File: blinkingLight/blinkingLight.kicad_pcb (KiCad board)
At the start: 2 copper layers, 50.8 x 50.8 mm, 11 parts, among them J1 Conn_02x03_Odd_Even, J2 Conn_01x02_Pin, Q1 BC548, U1 ICM7555xB

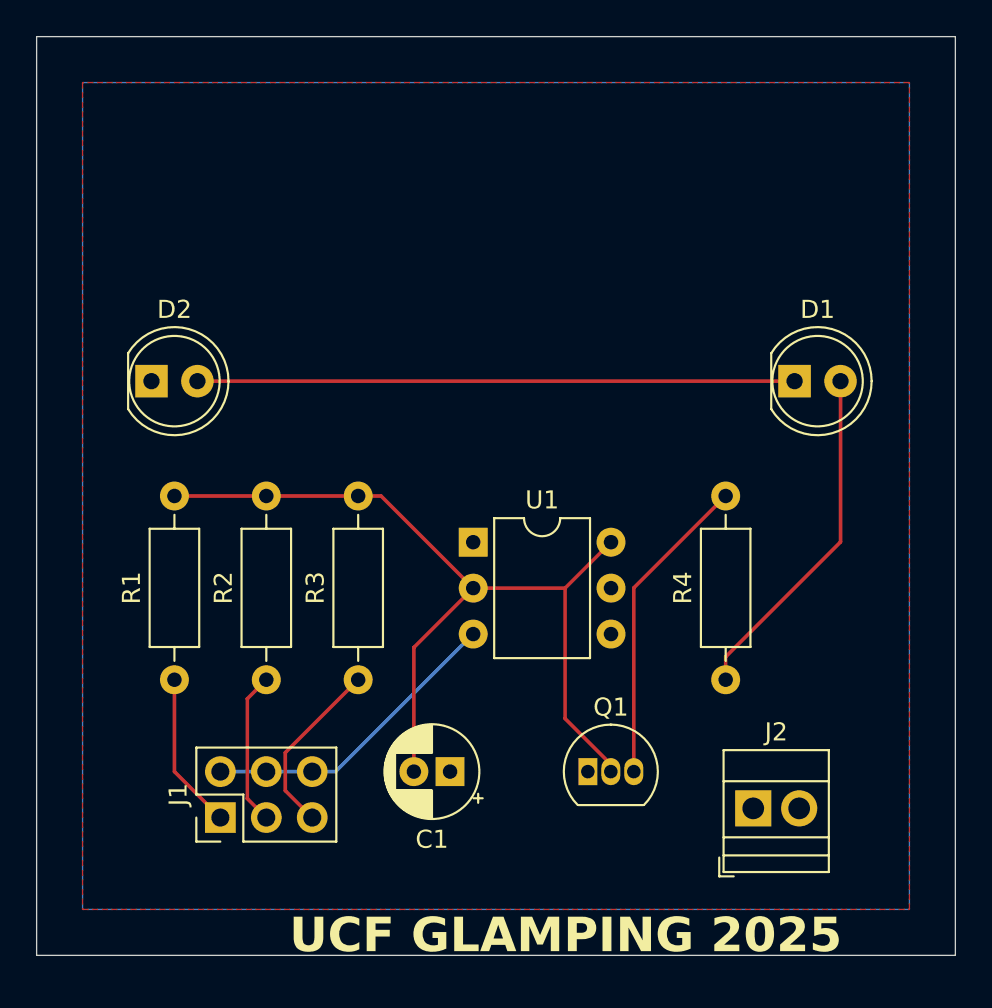
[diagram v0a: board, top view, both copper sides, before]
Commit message: fixed
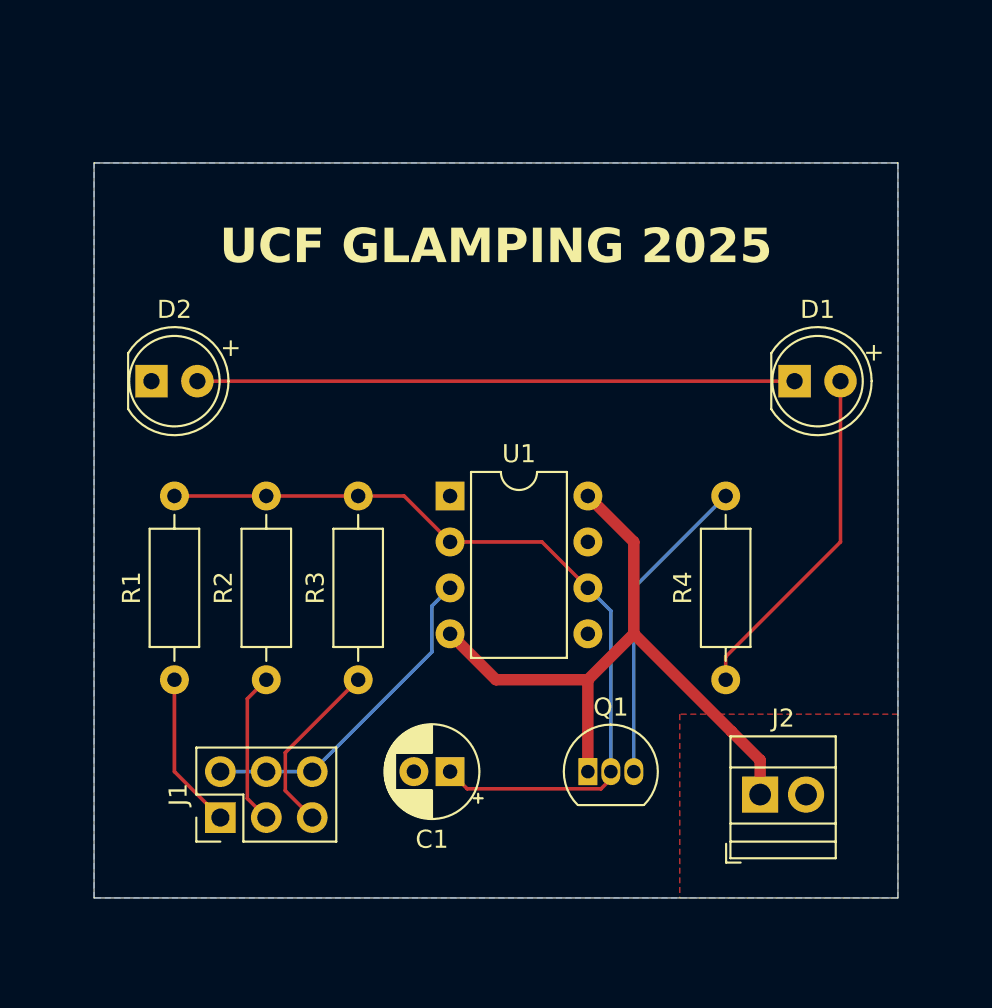
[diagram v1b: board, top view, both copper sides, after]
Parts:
- U1: footprint Package_DIP:DIP-6_W7.62mm -> Package_DIP:DIP-8_W7.62mm
- moved U1 2.86 mm to (124.5, 101.6)
- moved J2 0.85 mm to (141.6, 118.1)
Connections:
- C1 pad 1: GND -> Net-(Q1-B)
- C1 pad 2: Net-(Q1-B) -> GND
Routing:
- net +9V: track 0.00 -> 37.8 mm
- net Net-(Q1-B): track 50.0 -> 45.6 mm
- net Net-(J1-Pin_2): track 17.1 -> 18.4 mm
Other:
- board size 50.8 x 50.8 mm -> 44.4 x 40.6 mm
- board text added: "+"
